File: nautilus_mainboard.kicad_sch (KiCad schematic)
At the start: 4 parts

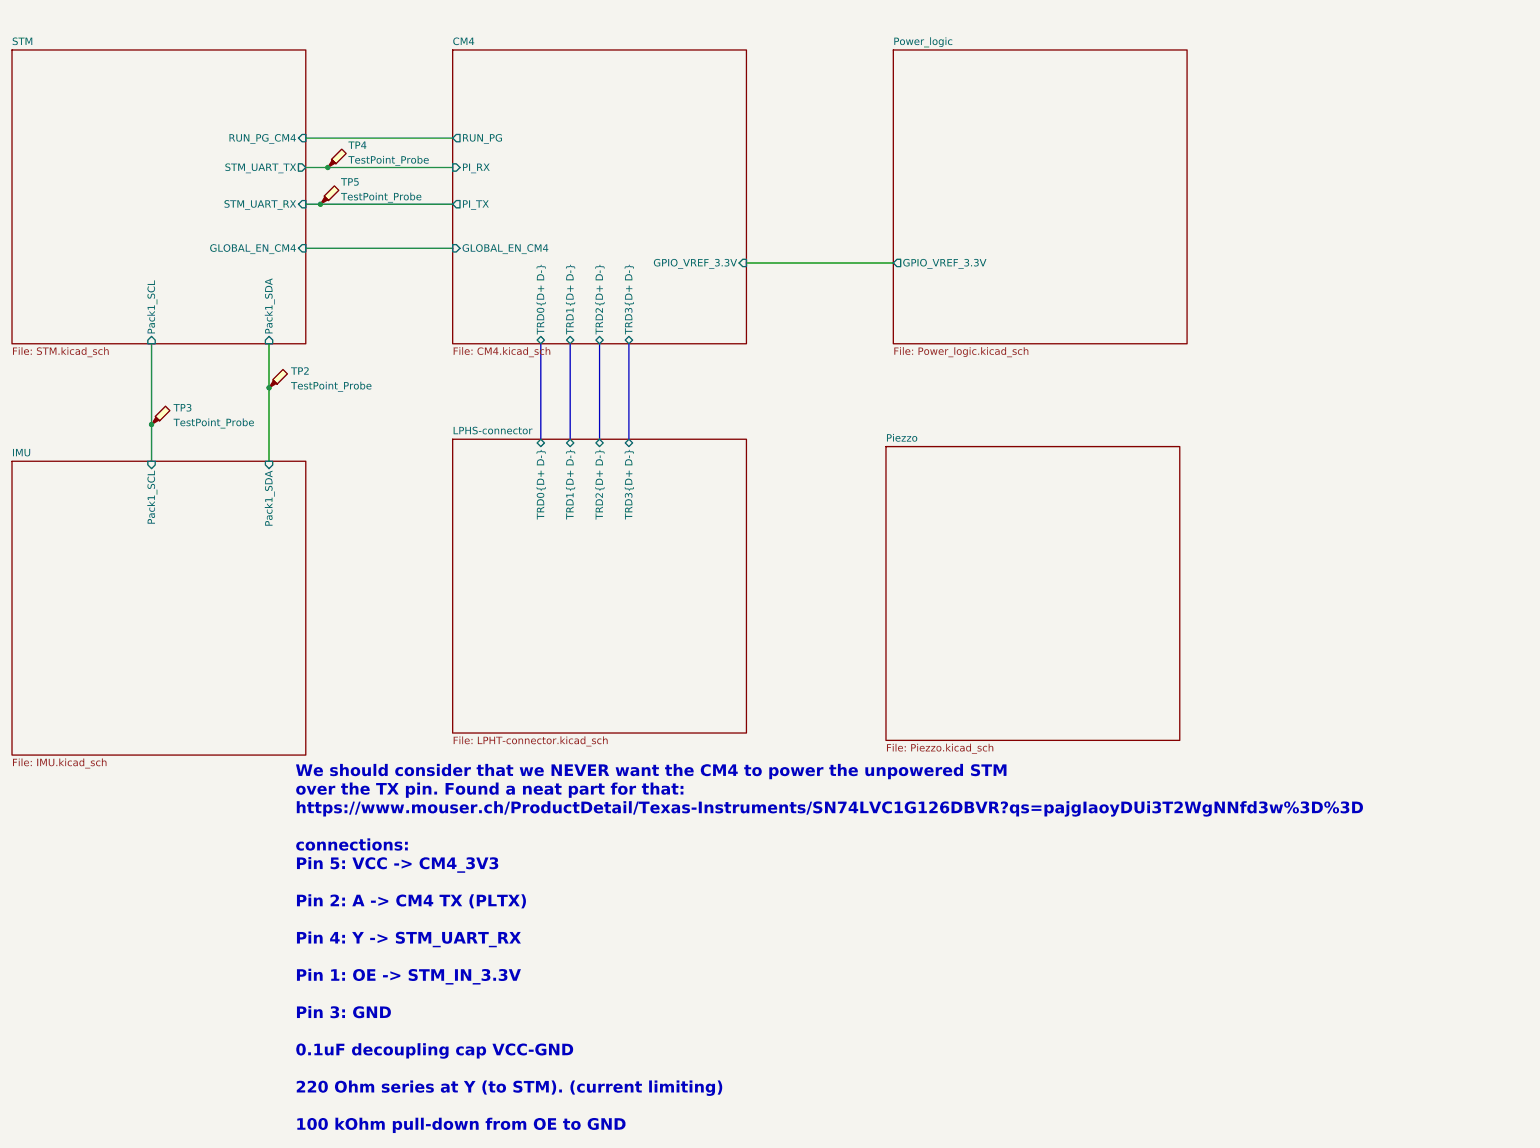
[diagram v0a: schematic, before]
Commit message: chore: Many routing changes
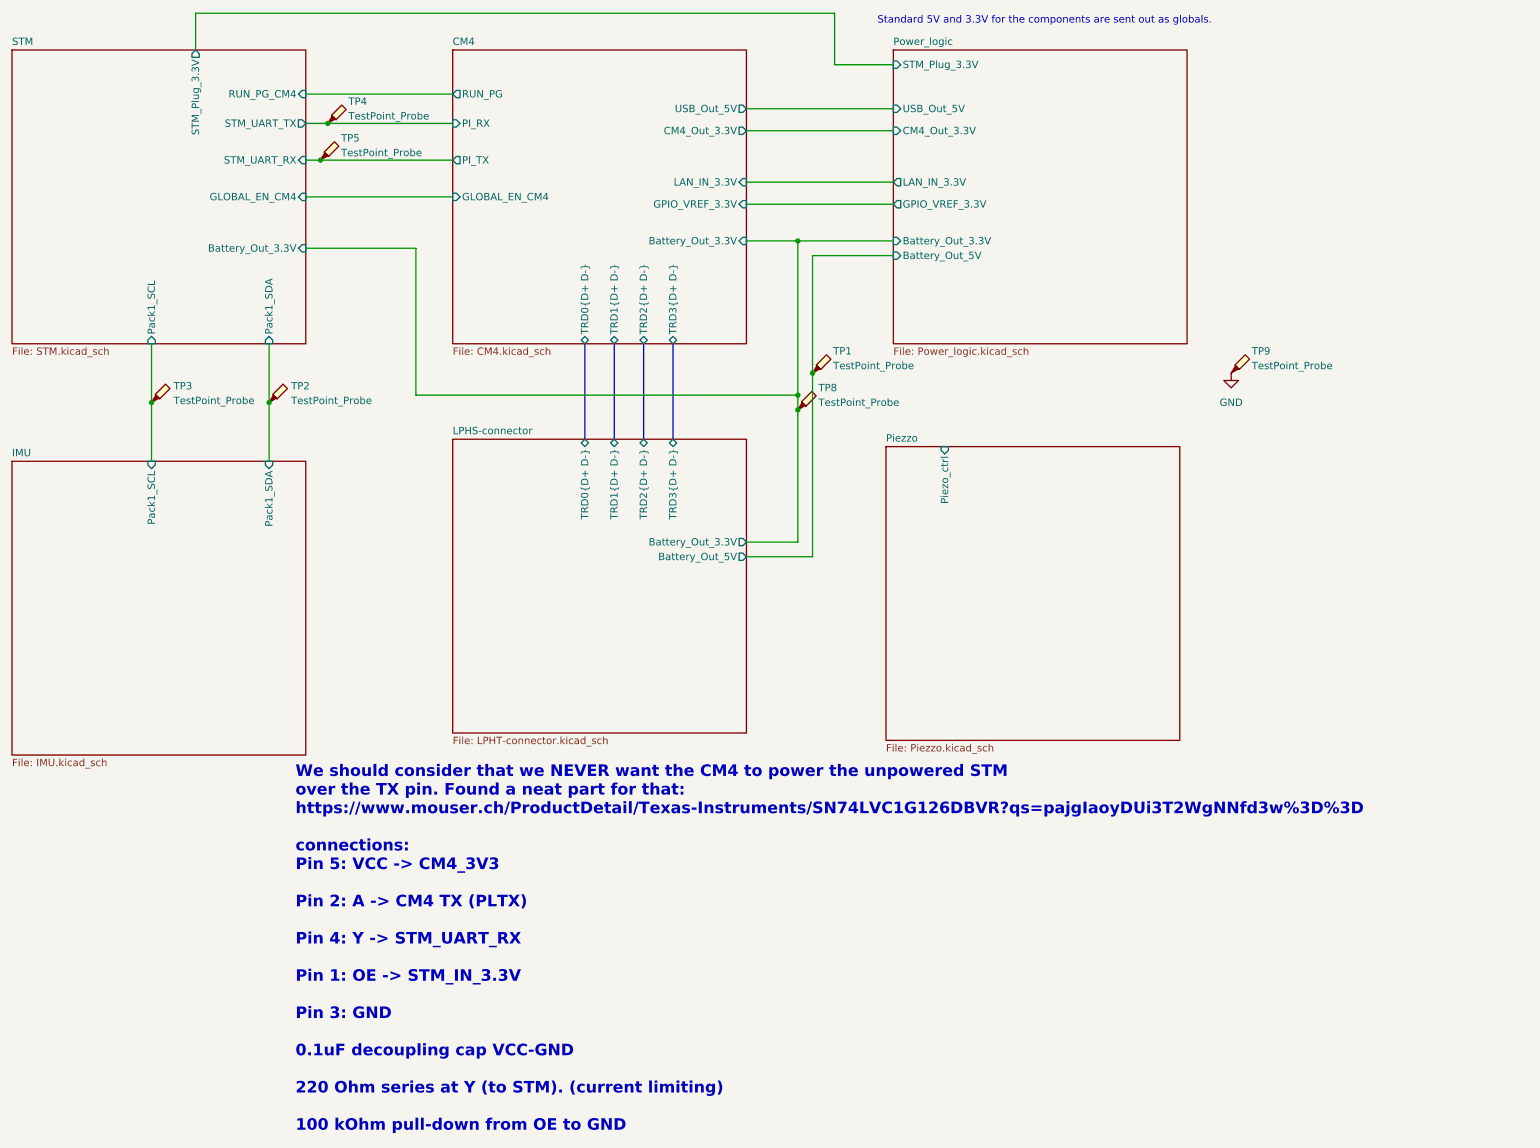
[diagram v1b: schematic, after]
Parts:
- added TP1, TP8, TP9: TestPoint_Probe, TestPoint:TestPoint_Pad_D1.0mm, symbol Connector:TestPoint_Probe
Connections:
- new net CM4/Battery_Out_3.3V: TP8.1
- new net GND: TP9.1
- new net LPHS-connector/Battery_Out_5V: TP1.1
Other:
- sheet CM4 ports: added Battery_Out_3.3V, CM4_Out_3.3V, LAN_IN_3.3V, USB_Out_5V; removed none
- sheet LPHS-connector ports: added Battery_Out_3.3V, Battery_Out_5V; removed none
- sheet Piezzo ports: added Piezo_ctrl; removed none
- sheet Power_logic ports: added Battery_Out_3.3V, Battery_Out_5V, CM4_Out_3.3V, LAN_IN_3.3V, STM_Plug_3.3V, USB_Out_5V; removed none
- sheet STM ports: added Battery_Out_3.3V, STM_Plug_3.3V; removed none
- note added: "Standard 5V and 3.3V for the components are sent out as globals."
- moved on the sheet: TP2, TP3, TP4, TP5
